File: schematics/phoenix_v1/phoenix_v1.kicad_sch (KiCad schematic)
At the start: 18 parts, among them J1 Screw_Terminal_01x02, J2 Conn_01x09_Socket, SW1 RotaryEncoder_Switch, U1 HHG1D-1, U2 ESP32-S3-DevKitC, U3 NHD-C0220BIZ

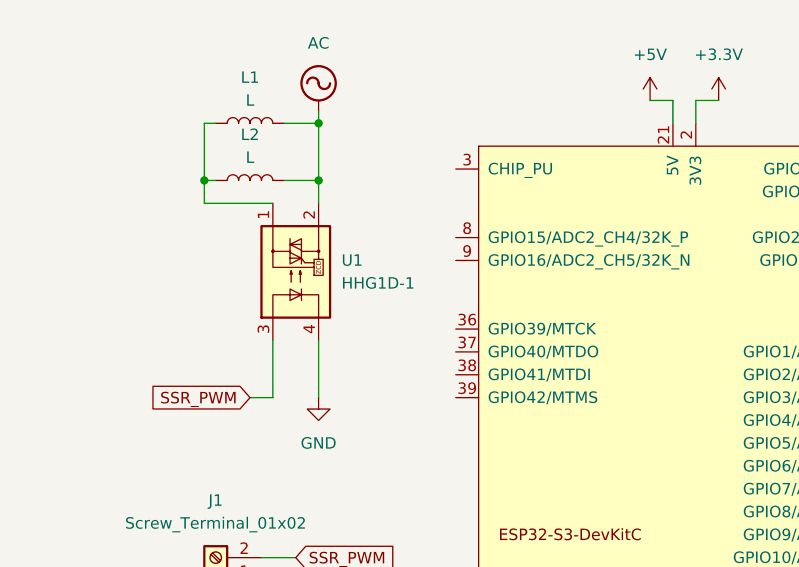
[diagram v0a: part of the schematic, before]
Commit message: tiny change to trigger diff
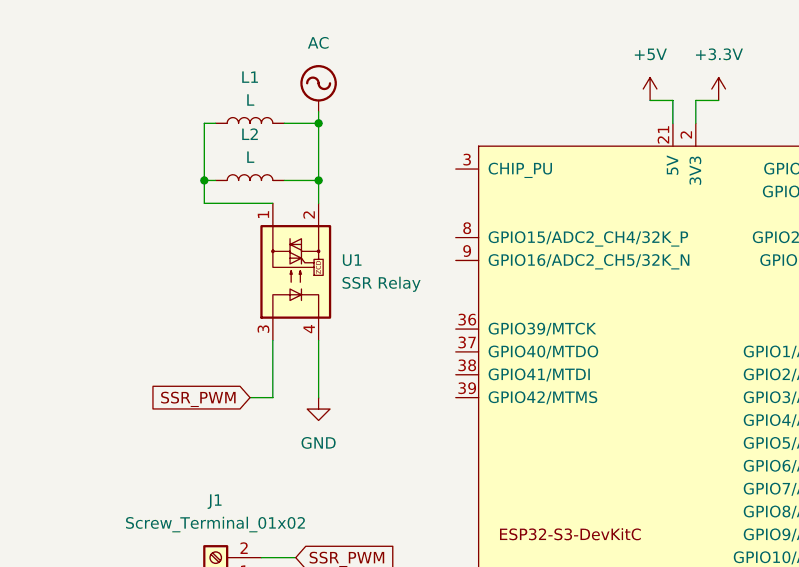
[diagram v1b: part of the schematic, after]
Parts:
- U1: value HHG1D-1 -> SSR Relay
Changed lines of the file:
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@@
 			)
 		)
-		(property "Value" "HHG1D-1"
+		(property "Value" "SSR Relay"
 			(at 55.88 63.4999 90)
 			(effects

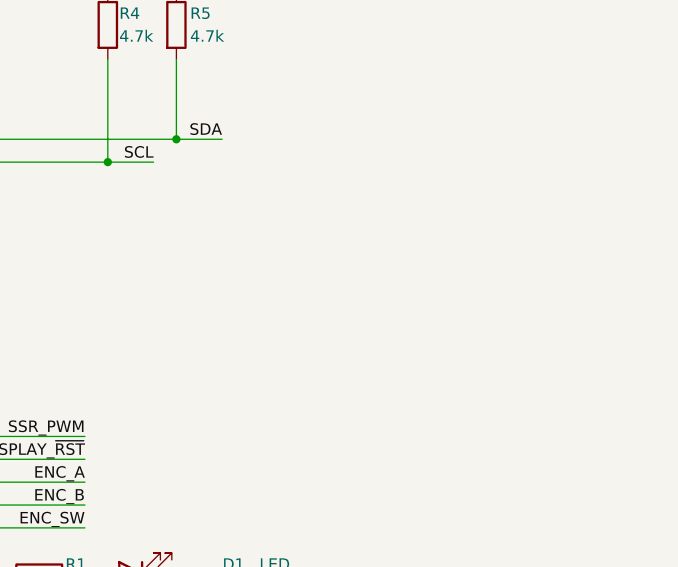
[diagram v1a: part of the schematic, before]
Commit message: another small diff
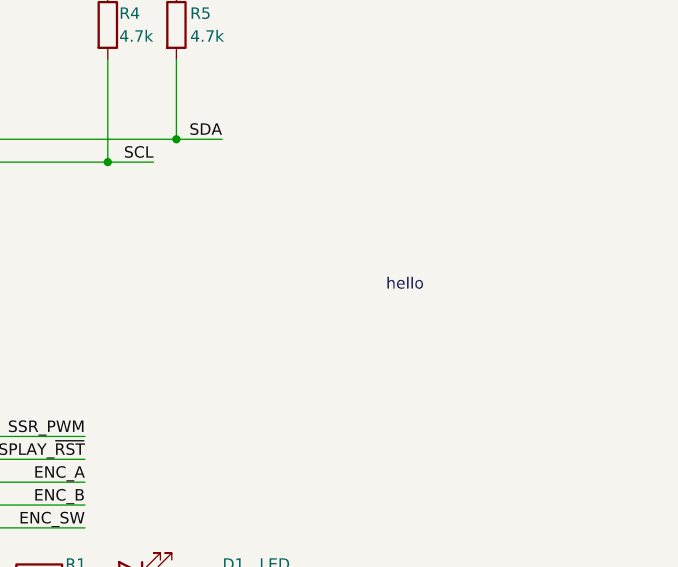
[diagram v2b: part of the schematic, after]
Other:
- note added: "hello"
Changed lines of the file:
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@@
+		)
+	)
+	(text "hello"
+		(exclude_from_sim no)
+		(at 167.64 94.996 0)
+		(effects
+			(font
+				(size 1.27 1.27)
+			)
 		)
 	)

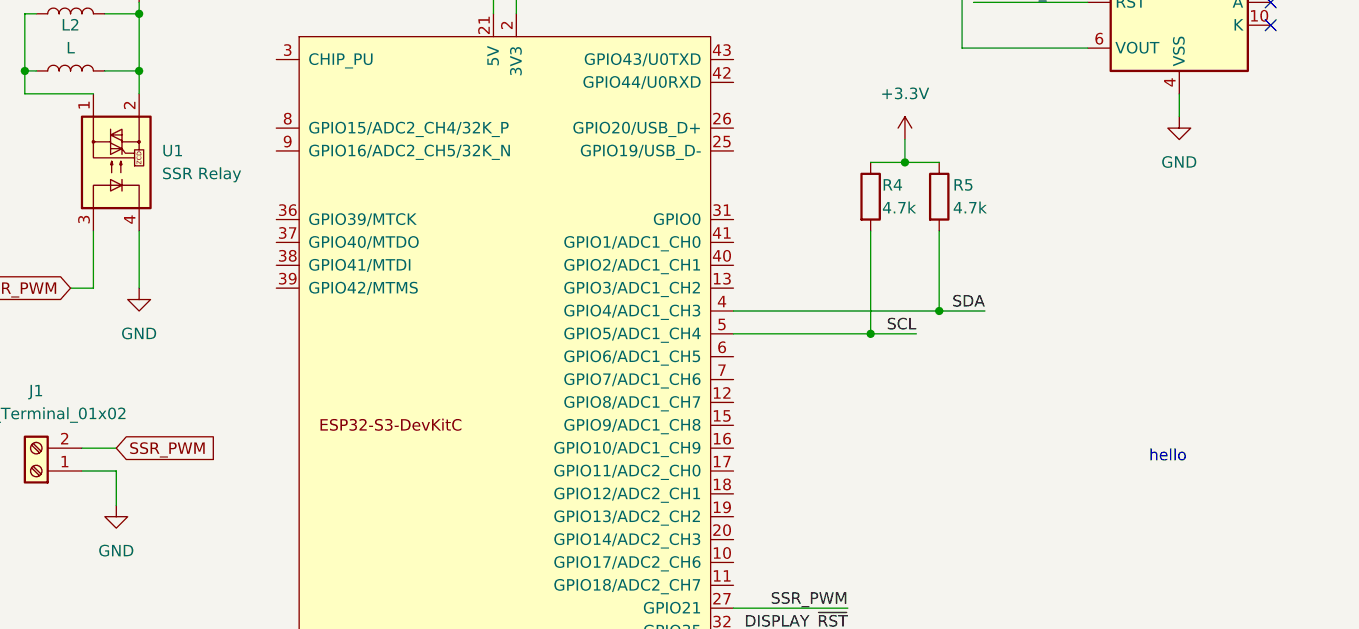
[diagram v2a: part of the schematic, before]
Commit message: delete random diff
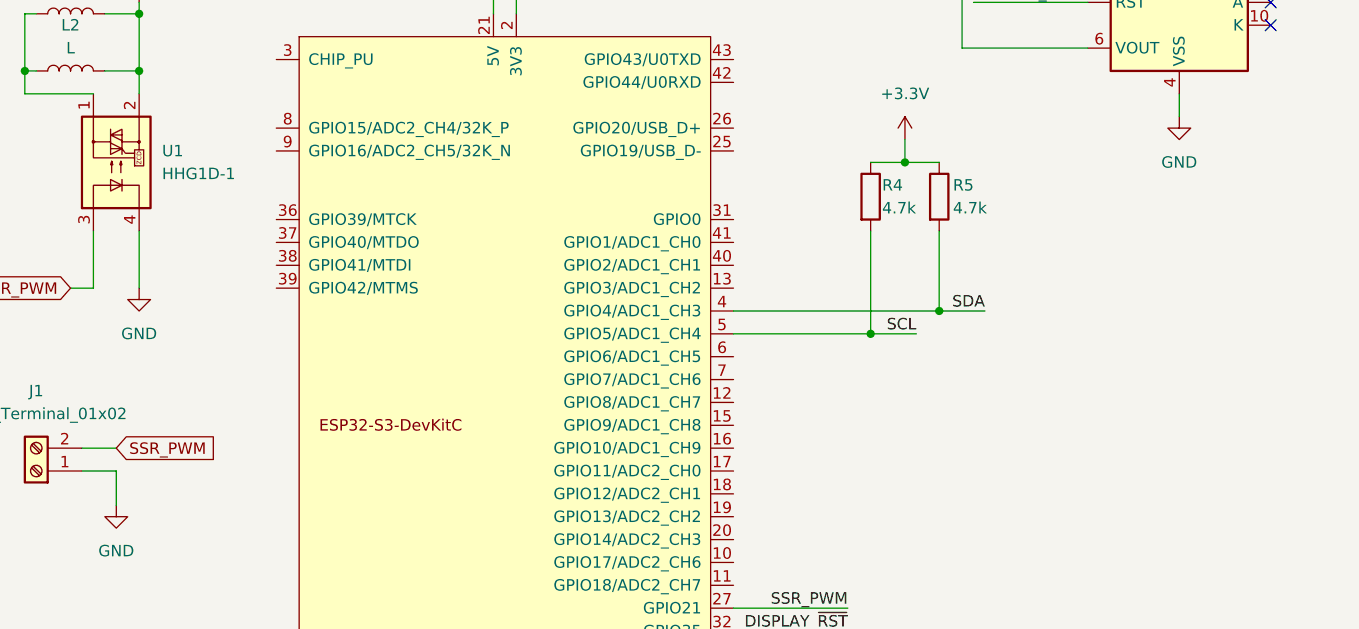
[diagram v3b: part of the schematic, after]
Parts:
- U1: value SSR Relay -> HHG1D-1
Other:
- note removed: "hello"
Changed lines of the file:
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@@
-		)
-	)
-	(text "hello"
-		(exclude_from_sim no)
-		(at 167.64 94.996 0)
-		(effects
-			(font
-				(size 1.27 1.27)
-			)
 		)
 	)
@@
 			)
 		)
-		(property "Value" "SSR Relay"
+		(property "Value" "HHG1D-1"
 			(at 55.88 63.4999 90)
 			(effects
